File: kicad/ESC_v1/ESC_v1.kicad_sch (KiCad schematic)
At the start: 41 parts, among them J1 Conn_01x05_Pin, J10 Conn_01x01_Pin, J11 Conn_01x01_Pin, J12 Conn_01x01_Pin, J13 Conn_01x03_Pin, J14 Conn_01x01_Pin, J15 Conn_01x01_Pin, J16 Conn_01x01_Pin, J17 Conn_01x02_Pin, J2 Conn_01x05_Pin, J3 Conn_01x03_Pin, J4 Conn_01x03_Pin, J5 Conn_01x05_Pin, J6 Conn_01x03_Pin, J7 Conn_01x04_Pin, J8 Conn_01x04_Pin, J9 Conn_01x02_Pin, U10 BD4104, U19 STM32G431CBUx, U7 ACS711xEXLT-15AB, U8 ACS711xEXLT-15AB

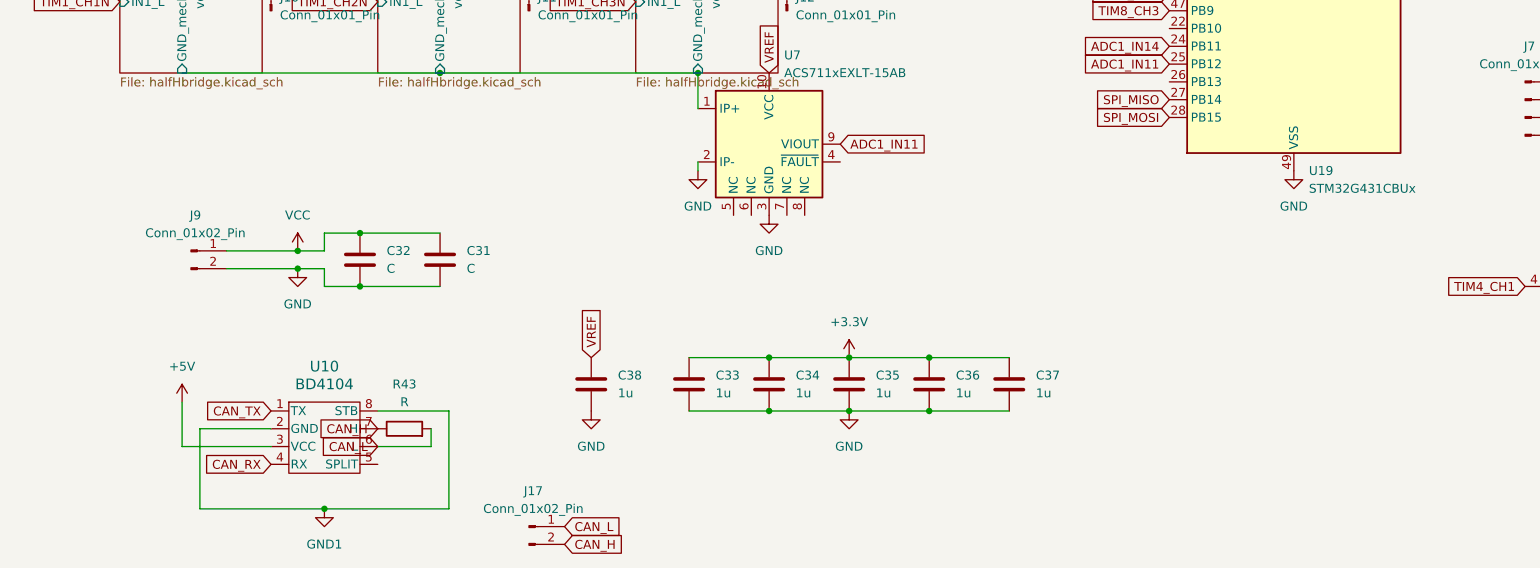
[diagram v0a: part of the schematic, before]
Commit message: a
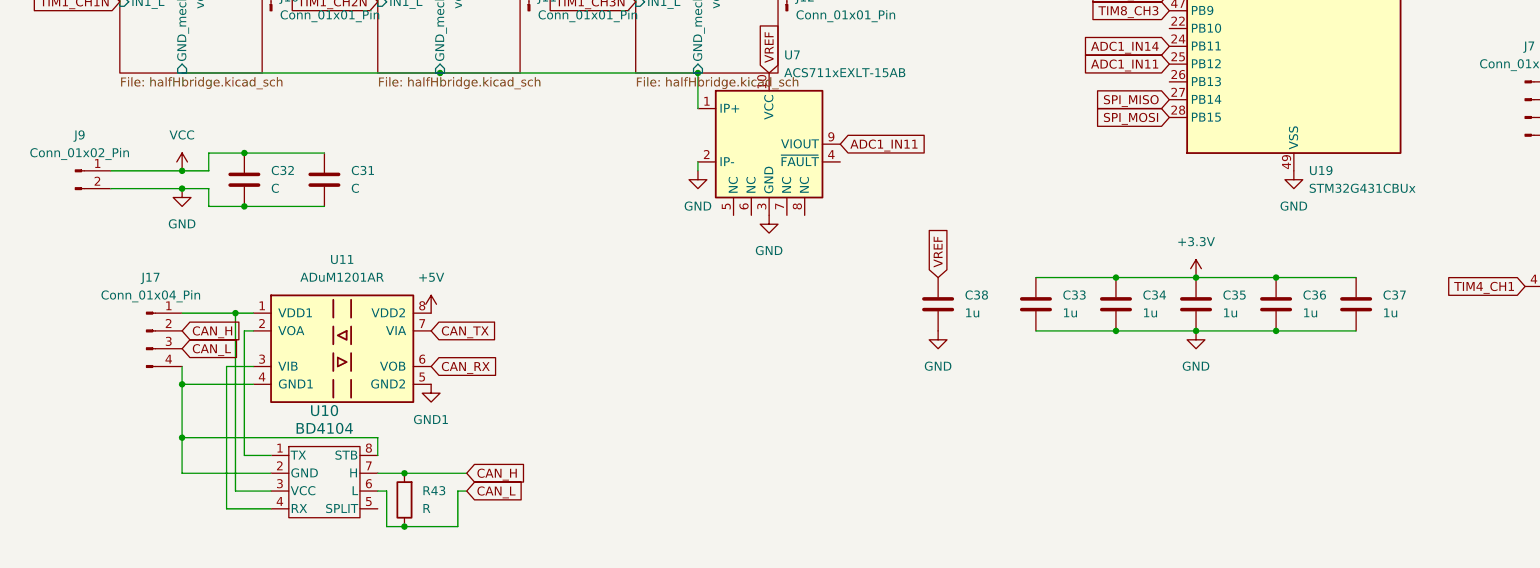
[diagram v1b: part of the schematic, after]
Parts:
- removed J17: Conn_01x02_Pin, symbol Connector:Conn_01x02_Pin
- added J17: Conn_01x04_Pin, Connector_JST:JST_PH_S4B-PH-K_1x04_P2.00mm_Horizontal, symbol Connector:Conn_01x04_Pin
- added U11: ADuM1201AR, Package_SO:SOIC-8_3.9x4.9mm_P1.27mm, symbol Isolator:ADuM1201AR
- J1, J2: footprint Connector_PinSocket_2.54mm:PinSocket_1x05_P2.54mm_Horizontal -> Connector_JST:JST_XH_S5B-XH-A_1x05_P2.50mm_Horizontal
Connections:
- net +5V: now also U11.8 (VDD2); no longer U10.3 (VCC)
- net CAN_H: now also R43.2, J17.2 (Pin_2); no longer R43.1
- net CAN_L: now also R43.1, J17.3 (Pin_3); no longer R43.2
- net CAN_RX: now also U11.6 (VOB); no longer U10.4 (RX)
- net CAN_TX: now also U11.7 (VIA); no longer U10.1 (TX)
- net GND1: now also U11.5 (GND2); no longer U10.2 (GND), U10.8 (STB)
- new net: J17.1 (Pin_1), U10.3 (VCC), U11.1 (VDD1)
- new net: U10.1 (TX), U11.2 (VOA)
- new net: U10.4 (RX), U11.3 (VIB)
- new net: J17.4 (Pin_4), U10.2 (GND), U10.8 (STB), U11.4 (GND1)
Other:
- moved on the sheet: C31, C32, C33, C34, C35, C36, C37, C38, J9, R43, U10
